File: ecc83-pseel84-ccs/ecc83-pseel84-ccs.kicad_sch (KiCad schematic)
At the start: 31 parts, among them Q1 DN2540N5-G, Q2 DN2540N5-G, T1 2,5 K, U1 ECC83, U2 LM317_TO-220, U3 EL84, U4 LM317_TO-220, U5 EL84

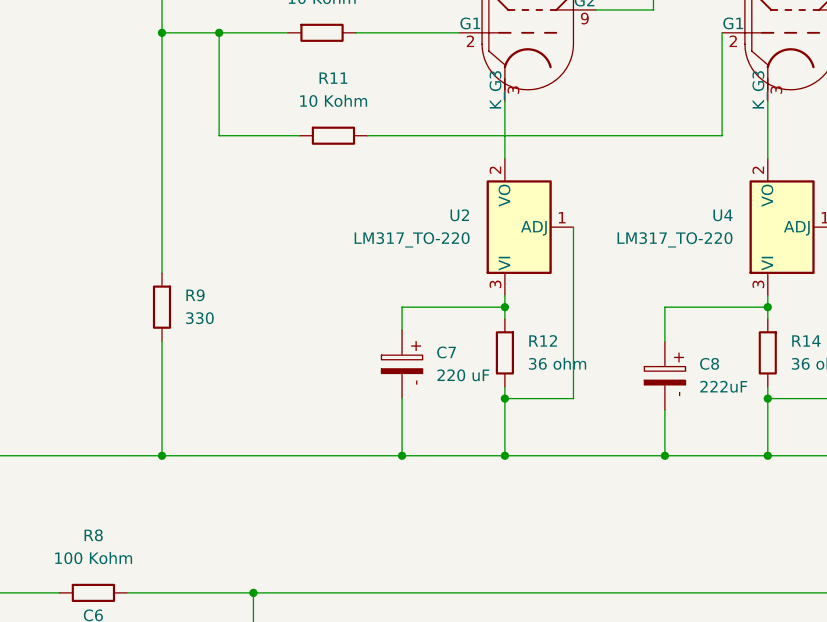
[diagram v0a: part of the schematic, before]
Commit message: princip scheman
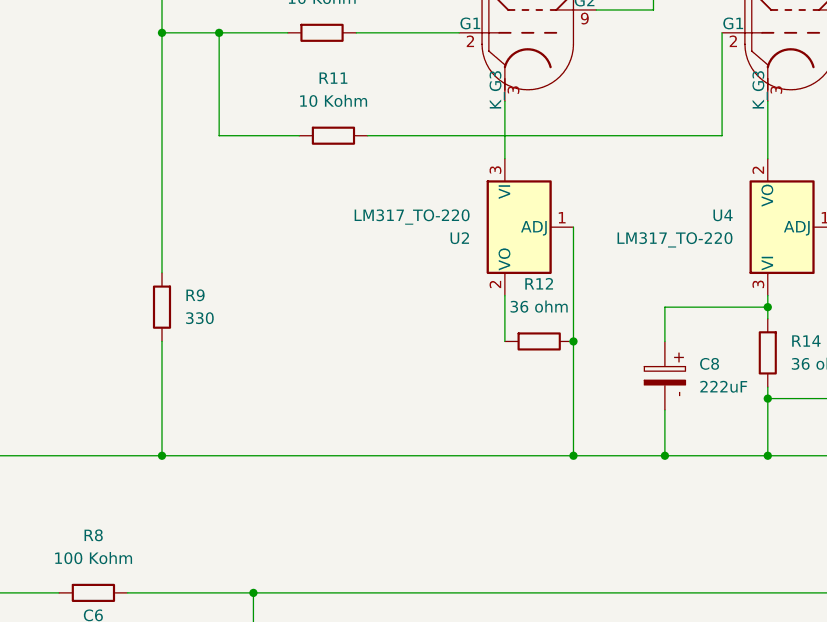
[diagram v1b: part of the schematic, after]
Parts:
- removed C7: 220 uF, Capacitor_THT:CP_Radial_D5.0mm_P2.00mm, symbol PCM_SL_Capacitors:22uF_50V
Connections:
- net at U3.3 (K_G3): now also U2.3 (VI); no longer U2.2 (VO)
- net at R12.1: now also U2.2 (VO); no longer U2.3 (VI)
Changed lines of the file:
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@@
 	)
 	(junction
-		(at 168.91 135.89)
+		(at 217.17 71.12)
 		(diameter 0)
 		(color 0 0 0 0)
 	)
 	(junction
-		(at 217.17 71.12)
+		(at 176.53 142.24)
 		(diameter 0)
 		(color 0 0 0 0)
@@
 	)
 	(junction
-		(at 157.48 142.24)
-		(diameter 0)
-		(color 0 0 0 0)
-	)
-	(junction
 		(at 107.95 157.48)
 		(diameter 0)
@@
 	)
 	(junction
-		(at 168.91 125.73)
-		(diameter 0)
-		(color 0 0 0 0)
-	)
-	(junction
 		(at 137.16 95.25)
 		(diameter 0)
@@
 	)
 	(junction
-		(at 186.69 142.24)
+		(at 176.53 129.54)
 		(diameter 0)
 		(color 0 0 0 0)
 	)
 	(junction
-		(at 168.91 142.24)
+		(at 186.69 142.24)
 		(diameter 0)
 		(color 0 0 0 0)
@@
 	(wire
 		(pts
-			(xy 130.81 142.24) (xy 157.48 142.24)
+			(xy 130.81 142.24) (xy 176.53 142.24)
 		)
 		(stroke
@@
 	(wire
 		(pts
-			(xy 168.91 135.89) (xy 168.91 142.24)
-		)
-		(stroke
-			(width 0)
-			(type default)
-		)
-	)
-	(wire
-		(pts
 			(xy 186.69 129.54) (xy 186.69 125.73)
 		)
@@
 	(wire
 		(pts
-			(xy 168.91 134.62) (xy 168.91 135.89)
+			(xy 210.82 142.24) (xy 256.54 142.24)
 		)
 		(stroke
@@
 	(wire
 		(pts
-			(xy 210.82 142.24) (xy 256.54 142.24)
+			(xy 176.53 142.24) (xy 186.69 142.24)
 		)
 		(stroke
@@
 	(wire
 		(pts
-			(xy 176.53 116.84) (xy 176.53 135.89)
+			(xy 176.53 116.84) (xy 176.53 129.54)
 		)
 		(stroke
@@
 	(wire
 		(pts
-			(xy 176.53 135.89) (xy 168.91 135.89)
-		)
-		(stroke
-			(width 0)
-			(type default)
-		)
-	)
-	(wire
-		(pts
 			(xy 171.45 82.55) (xy 171.45 76.2)
 		)
@@
 	(wire
 		(pts
-			(xy 157.48 135.89) (xy 157.48 142.24)
-		)
-		(stroke
-			(width 0)
-			(type default)
-		)
-	)
-	(wire
-		(pts
-			(xy 168.91 127) (xy 168.91 125.73)
-		)
-		(stroke
-			(width 0)
-			(type default)
-		)
-	)
-	(wire
-		(pts
-			(xy 157.48 142.24) (xy 168.91 142.24)
+			(xy 176.53 129.54) (xy 176.53 142.24)
 		)
 		(stroke
@@
 	(wire
 		(pts
-			(xy 157.48 125.73) (xy 168.91 125.73)
+			(xy 36.83 142.24) (xy 64.77 142.24)
 		)
 		(stroke
@@
 	(wire
 		(pts
-			(xy 36.83 142.24) (xy 64.77 142.24)
+			(xy 57.15 100.33) (xy 59.69 100.33)
 		)
 		(stroke
@@
 	(wire
 		(pts
-			(xy 57.15 100.33) (xy 59.69 100.33)
+			(xy 82.55 60.96) (xy 82.55 64.77)
 		)
 		(stroke
@@
 	(wire
 		(pts
-			(xy 82.55 60.96) (xy 82.55 64.77)
+			(xy 168.91 124.46) (xy 168.91 129.54)
 		)
 		(stroke
@@
 	(wire
 		(pts
-			(xy 168.91 142.24) (xy 186.69 142.24)
-		)
-		(stroke
-			(width 0)
-			(type default)
-		)
-	)
-	(wire
-		(pts
 			(xy 67.31 86.36) (xy 115.57 86.36)
 		)
@@
 	(wire
 		(pts
-			(xy 157.48 128.27) (xy 157.48 125.73)
-		)
-		(stroke
-			(width 0)
-			(type default)
-		)
-	)
-	(wire
-		(pts
 			(xy 193.04 95.25) (xy 193.04 106.68)
 		)
@@
 	(wire
 		(pts
-			(xy 168.91 125.73) (xy 168.91 124.46)
-		)
-		(stroke
-			(width 0)
-			(type default)
-		)
-	)
-	(wire
-		(pts
 			(xy 256.54 76.2) (xy 266.7 76.2)
 		)
@@
 		(lib_id "Regulator_Linear:LM317_TO-220")
 		(at 168.91 116.84 90)
+		(mirror x)
 		(unit 1)
 		(exclude_from_sim no)
@@
 		(on_board yes)
 		(dnp no)
-		(fields_autoplaced yes)
 		(property "Reference" "U2"
-			(at 165.1 115.5699 90)
+			(at 165.1 118.1101 90)
 			(effects
 				(font
@@
 		)
 		(property "Value" "LM317_TO-220"
-			(at 165.1 118.1099 90)
+			(at 165.1 115.5701 90)
 			(effects
 				(font
@@
 	)
 	(symbol
+		(lib_id "PCM_SL_Resistors:470ohm")
+		(at 172.72 129.54 0)
+		(unit 1)
+		(exclude_from_sim no)
+		(in_bom yes)
+		(on_board yes)
+		(dnp no)
+		(fields_autoplaced yes)
+		(property "Reference" "R12"
+			(at 172.72 123.19 0)
+			(effects
+				(font
+					(size 1.27 1.27)
+				)
+			)
+		)
+		(property "Value" "36 ohm"
+			(at 172.72 125.73 0)
+			(effects
+				(font
+					(size 1.27 1.27)
+				)
+			)
+		)
+		(property "Footprint" "Resistor_THT:R_Axial_DIN0207_L6.3mm_D2.5mm_P10.16mm_Horizontal"
+			(at 173.609 133.858 0)
+			(effects
+				(font
+					(size 1.27 1.27)
+				)
+				(hide yes)
+			)
+		)
+		(property "Datasheet" ""
+			(at 173.228 129.54 0)
+			(effects
+				(font
+					(size 1.27 1.27)
+				)
+				(hide yes)
+			)
+		)
+		(property "Description" "470Ω, 1/4W Resistor"
+			(at 172.72 129.54 0)
+			(effects
+				(font
+					(size 1.27 1.27)
+				)
+				(hide yes)
+			)
+		)
+		(pin "1"
+		)
+		(pin "2"
+		)
+		(instances
+			(project "ecc83-pseel84-ccs"
+				(path "/ede9bcd0-3b88-45ca-8857-ae16dd120ce1"
+					(reference "R12")
+					(unit 1)
+				)
+			)
+		)
+	)
+	(symbol
 		(lib_id "power:Earth")
 		(at 210.82 148.59 0)
@@
 					(unit 1)
 				)
-			)
-		)
-	)
-	(symbol
-		(lib_id "PCM_SL_Capacitors:22uF_50V")
-		(at 157.48 132.08 270)
-		(unit 1)
-		(exclude_from_sim no)
-		(in_bom yes)
-		(on_board yes)
-		(dnp no)
-		(fields_autoplaced yes)
-		(property "Reference" "C7"
-			(at 161.29 130.8099 90)
-			(effects
-				(font
-					(size 1.27 1.27)
-				)
-				(justify left)
-			)
-		)
-		(property "Value" "220 uF"
-			(at 161.29 133.3499 90)
-			(effects
-				(font
-					(size 1.27 1.27)
-				)
-				(justify left)
-			)
-		)
-		(property "Footprint" "Capacitor_THT:CP_Radial_D5.0mm_P2.00mm"
-			(at 153.67 132.842 0)
-			(effects
-				(font
-					(size 1.27 1.27)
-				)
-				(hide yes)
-			)
-		)
-		(property "Datasheet" ""
-			(at 157.48 132.588 0)
-			(effects
-				(font
-					(size 1.27 1.27)
-				)
-				(hide yes)
-			)
-		)
-		(property "Description" "22uF, 50V Electrolytic Capacitor"
-			(at 157.48 132.08 0)
-			(effects
-				(font
-					(size 1.27 1.27)
-				)
-				(hide yes)
-			)
-		)
-		(pin "2"
-		)
-		(pin "1"
-		)
-		(instances
-			(project "ecc83-pseel84-ccs"
-				(path "/ede9bcd0-3b88-45ca-8857-ae16dd120ce1"
-					(reference "C7")
-					(unit 1)
-				)
-			)
-		)
-	)
-	(symbol
-		(lib_id "PCM_SL_Resistors:470ohm")
-		(at 168.91 130.81 270)
-		(unit 1)
-		(exclude_from_sim no)
-		(in_bom yes)
-		(on_board yes)
-		(dnp no)
-		(fields_autoplaced yes)
-		(property "Reference" "R12"
-			(at 171.45 129.5399 90)
-			(effects
-				(font
-					(size 1.27 1.27)
-				)
-				(justify left)
-			)
-		)
-		(property "Value" "36 ohm"
-			(at 171.45 132.0799 90)
-			(effects
-				(font
-					(size 1.27 1.27)
-				)
-				(justify left)
-			)
-		)
-		(property "Footprint" "Resistor_THT:R_Axial_DIN0207_L6.3mm_D2.5mm_P10.16mm_Horizontal"
-			(at 164.592 131.699 0)
-			(effects
-				(font
-					(size 1.27 1.27)
-				)
-				(hide yes)
-			)
-		)
-		(property "Datasheet" ""
-			(at 168.91 131.318 0)
-			(effects
-				(font
-					(size 1.27 1.27)
-				)
-				(hide yes)
-			)
-		)
-		(property "Description" "470Ω, 1/4W Resistor"
-			(at 168.91 130.81 0)
-			(effects
-				(font
-					(size 1.27 1.27)
-				)
-				(hide yes)
-			)
-		)
-		(pin "1"
-		)
-		(pin "2"
-		)
-		(instances
-			(project "ecc83-pseel84-ccs"
-				(path "/ede9bcd0-3b88-45ca-8857-ae16dd120ce1"
-					(reference "R12")
-					(unit 1)
-				)
